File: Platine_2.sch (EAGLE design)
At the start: 19 parts, among them X2 DTF13-12PA

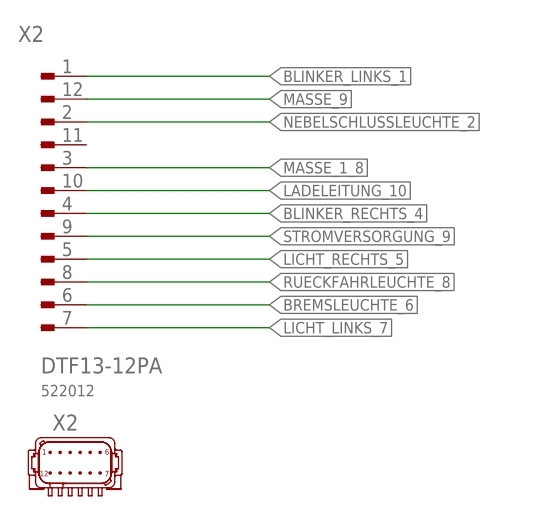
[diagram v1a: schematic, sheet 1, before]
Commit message: Diode added !
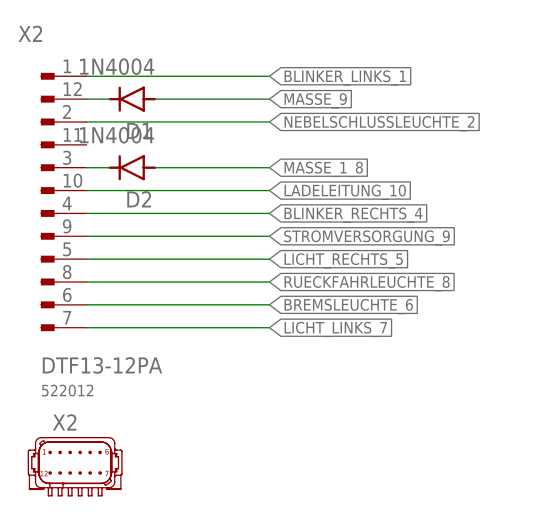
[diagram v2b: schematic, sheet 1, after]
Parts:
- added D1, D2: 1N4004, Diodes:1N4004
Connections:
- new net N$10: D1.C, X2G$1.12
- new net N$11: D2.C, X2G$1.3
- net MASSE_1_8: now also D2.A; no longer X2G$1.3
- net MASSE_9: now also D1.A; no longer X2G$1.12
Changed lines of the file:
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@@
 <part name="FRAME1" library="frames" library_urn="urn:adsk.eagle:library:229" deviceset="A4P-LOC" device=""/>
 <part name="FRAME2" library="frames" library_urn="urn:adsk.eagle:library:229" deviceset="A4P-LOC" device=""/>
+<part name="D1" library="Diodes" library_urn="urn:adsk.eagle:library:11396254" deviceset="1N4004" device="" package3d_urn="urn:adsk.eagle:package:10898391/4"/>
+<part name="D2" library="Diodes" library_urn="urn:adsk.eagle:library:11396254" deviceset="1N4004" device="" package3d_urn="urn:adsk.eagle:package:10898391/4"/>
 </parts>
 <sheets>
@@
 <attribute name="LAST_DATE_TIME" x="140.97" y="10.16" size="2.286" layer="94"/>
 <attribute name="SHEET" x="154.305" y="5.08" size="2.54" layer="94"/>
+</instance>
+<instance part="D1" gate="G$1" x="27.94" y="63.5" smashed="yes" rot="R180">
+<attribute name="NAME" x="30.2514" y="60.8584" size="1.778" layer="95" rot="R180"/>
+<attribute name="VALUE" x="30.5054" y="67.9958" size="1.778" layer="96" rot="R180"/>
+</instance>
+<instance part="D2" gate="G$1" x="27.94" y="55.88" smashed="yes" rot="R180">
+<attribute name="NAME" x="30.2514" y="53.2384" size="1.778" layer="95" rot="R180"/>
+<attribute name="VALUE" x="30.5054" y="60.3758" size="1.778" layer="96" rot="R180"/>
 </instance>
 </instances>
@@
 <net name="MASSE_1_8" class="0">
 <segment>
-<pinref part="X2" gate="G$1" pin="3"/>
-<wire x1="22.86" y1="55.88" x2="43.18" y2="55.88" width="0.1524" layer="91"/>
 <label x="43.18" y="55.88" size="1.27" layer="95" xref="yes"/>
+<wire x1="30.48" y1="55.88" x2="43.18" y2="55.88" width="0.1524" layer="91"/>
+<pinref part="D2" gate="G$1" pin="A"/>
 </segment>
 </net>
 <net name="MASSE_9" class="0">
 <segment>
-<pinref part="X2" gate="G$1" pin="12"/>
-<wire x1="22.86" y1="63.5" x2="43.18" y2="63.5" width="0.1524" layer="91"/>
 <label x="43.18" y="63.5" size="1.27" layer="95" xref="yes"/>
+<wire x1="30.48" y1="63.5" x2="43.18" y2="63.5" width="0.1524" layer="91"/>
+<pinref part="D1" gate="G$1" pin="A"/>
 </segment>
 </net>
+<net name="N$10" class="0">
+<segment>
+<pinref part="X2" gate="G$1" pin="12"/>
+<wire x1="22.86" y1="63.5" x2="25.4" y2="63.5" width="0.1524" layer="91"/>
+<pinref part="D1" gate="G$1" pin="C"/>
+</segment>
+</net>
+<net name="N$11" class="0">
+<segment>
+<pinref part="X2" gate="G$1" pin="3"/>
+<wire x1="22.86" y1="55.88" x2="25.4" y2="55.88" width="0.1524" layer="91"/>
+<pinref part="D2" gate="G$1" pin="C"/>
+</segment>
+</net>
